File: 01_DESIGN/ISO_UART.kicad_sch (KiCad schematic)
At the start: 3 parts, among them U7 ISO7721DR

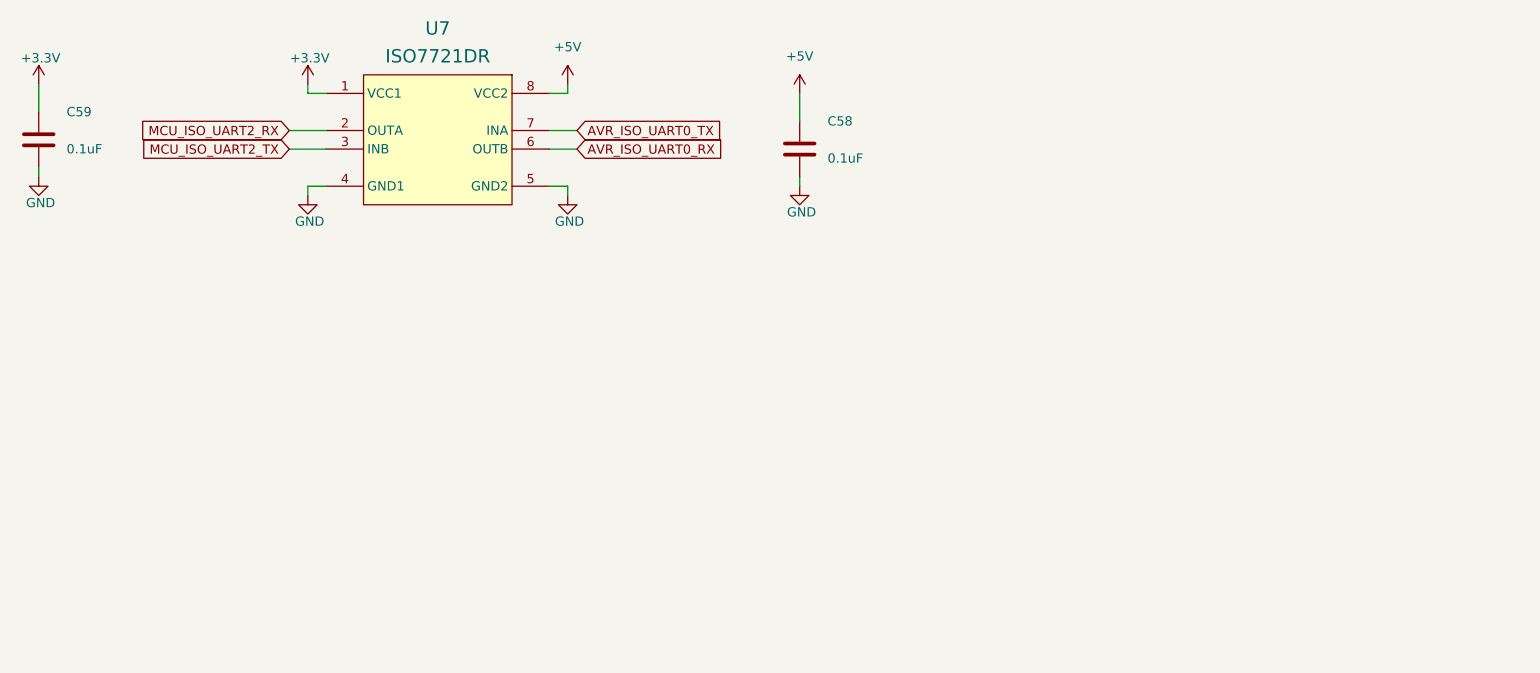
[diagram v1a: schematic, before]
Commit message: Update KiCad project files
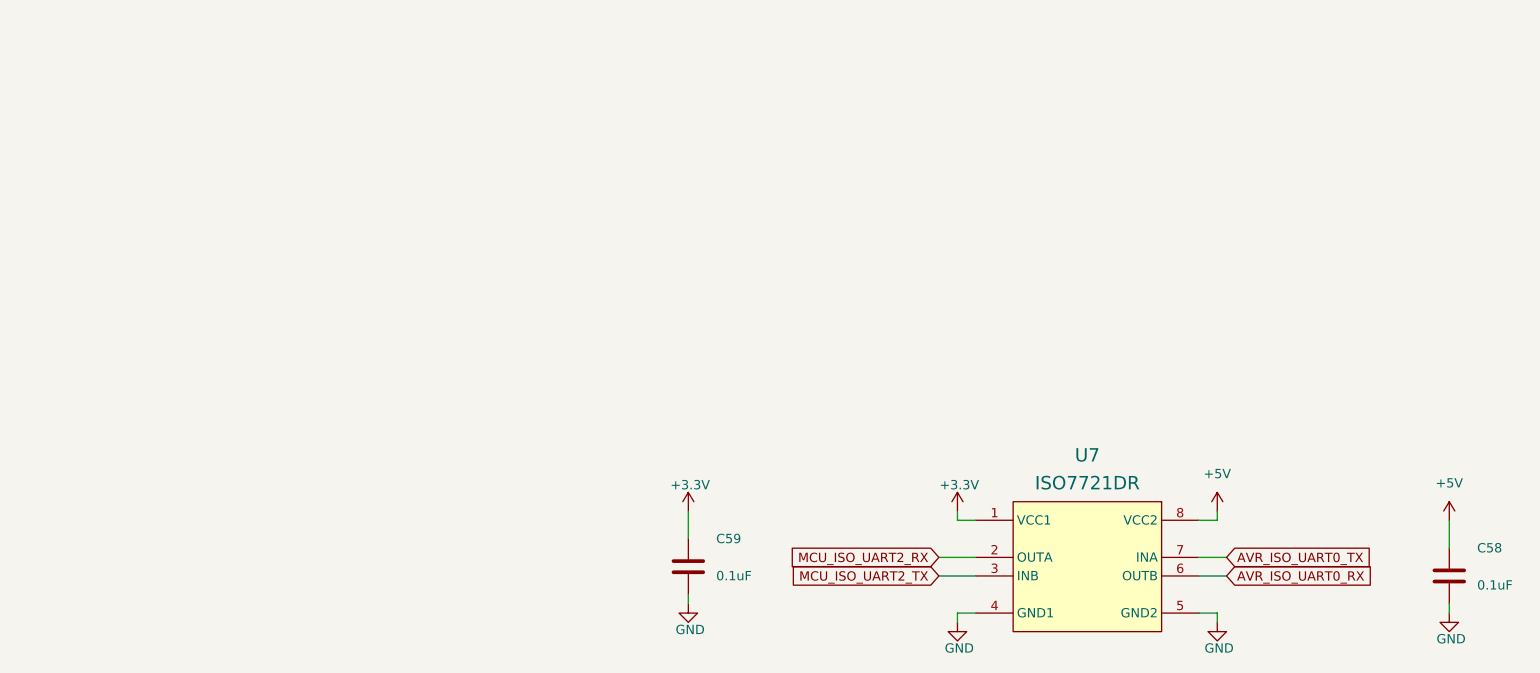
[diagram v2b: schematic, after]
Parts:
- C58, C59: symbol Device:C -> LABLIB:C
- U7: symbol AUSB:ISO7721DR -> LABLIB:ISO7721DR
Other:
- moved on the sheet: C58, C59, U7
